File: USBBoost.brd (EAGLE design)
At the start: 43.8 x 20.3 mm, 27 parts, among them IC1 RT9276, J1 Input, J2 3.75V, J3 2.33V, J4 1.17V, J5 Status, X1 USB_

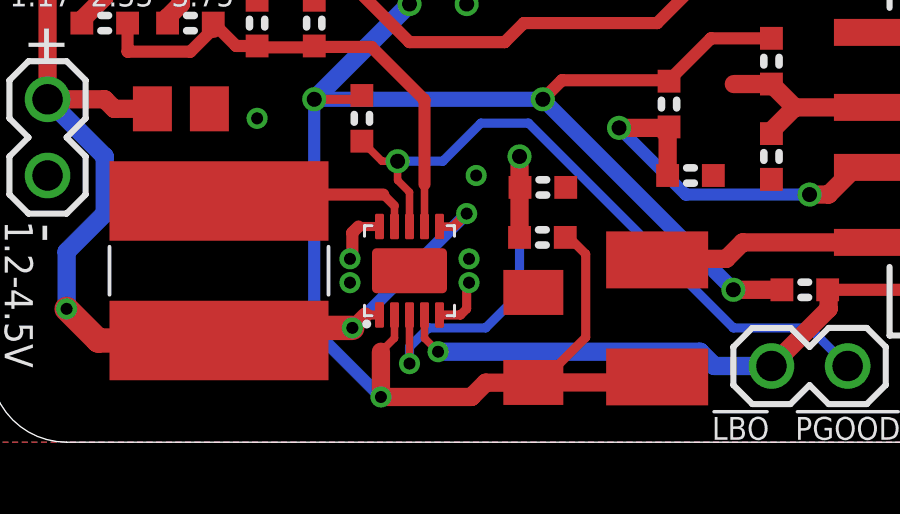
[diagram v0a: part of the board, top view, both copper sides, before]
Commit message: foo
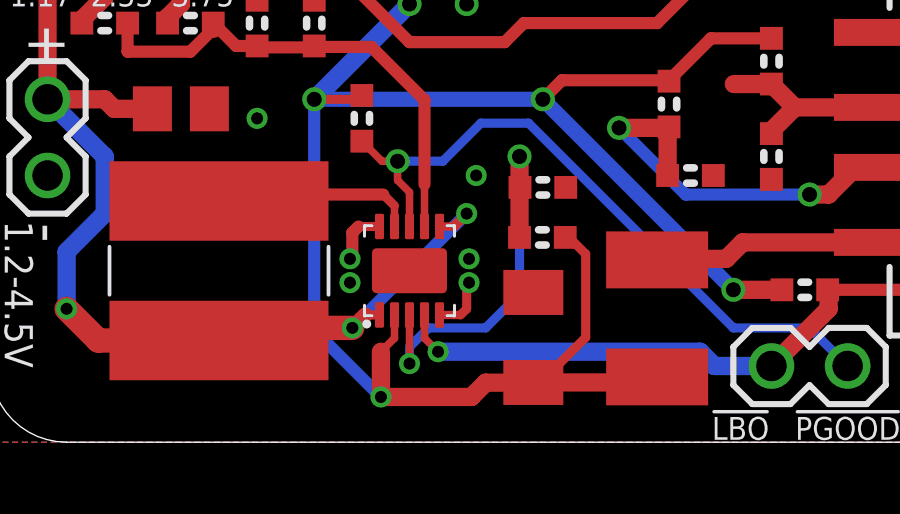
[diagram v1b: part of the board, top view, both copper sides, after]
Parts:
- removed R15: 20k0, freetronics-original:0603
- added R3: 49k9, freetronics-original:0603
- R10: value 1k -> 130k
- R11: value 130k -> 73k2
- R12: value 73k2 -> 26k7
- R13: value 26k7 -> 20k
- R14: value 20k -> 20k0
- R5: value 49k9 -> 180k
- R6: value 180k -> 10k
- R8: value 10k -> 1k
- moved R8 17.0 mm to (15.9, 17.8), turned to 90 degrees
- moved R7 15.8 mm to (27.1, 5.08), turned to 0 degrees
- moved R14 9.38 mm to (18.4, 8.49), turned to 180 degrees
- moved R5 8.10 mm to (18.4, 6.83), turned to 180 degrees
- moved R6 7.21 mm to (12.4, 10.8), turned to 270 degrees
- moved R13 6.98 mm to (10.8, 14.0), turned to 270 degrees
- moved R10 6.35 mm to (8.89, 14.0)
- moved R12 2.86 mm to (3.81, 14.0)
- moved R4 2.77 mm to (26.0, 9.53), turned to 270 degrees
- moved R11 2.22 mm to (6.67, 14.0), turned to 180 degrees
- moved R9 1.90 mm to (14.0, 17.8)
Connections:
- net !LBO: now also R7.2; no longer R8.2
- net !PGOOD: now also R6.2; no longer R7.2
- net FB: now also R14.2, R5.2; no longer R15.2, R6.2
- net GND: now also R13.1, R3.2; no longer R15.1, R5.2
- net LBI: now also R10.1, R13.2; no longer R13.1, R14.2
- net N$10: now also R4.1; no longer R5.1
- net N$11: now also R11.2; no longer R12.2
- net N$12: now also R12.2; no longer R13.2
- net N$15: now also R9.2; no longer R10.2
- net N$5: now also R10.2; no longer R11.2
- net N$7: now also R3.1; no longer R4.1
- net N$8: now also R8.2; no longer R9.2
- net VOUT: now also R5.1; no longer R10.1
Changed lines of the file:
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@@
 <elements>
 <element name="C1" library="freetronics-jon" package="C0805" value="10uF" x="6.35" y="11.1125" smashed="yes"/>
-<element name="R15" library="freetronics-original" package="0603" value="20k0" x="18.415" y="8.493125" smashed="yes" rot="R180"/>
-<element name="R6" library="freetronics-original" package="0603" value="180k" x="18.399225" y="6.82625" smashed="yes" rot="R180"/>
+<element name="R14" library="freetronics-original" package="0603" value="20k0" x="18.415" y="8.493125" smashed="yes" rot="R180"/>
+<element name="R5" library="freetronics-original" package="0603" value="180k" x="18.399225" y="6.82625" smashed="yes" rot="R180"/>
 <element name="C2" library="freetronics-jon" package="C1206K" value="22uF" x="18.0975" y="3.4924" smashed="yes" rot="R90"/>
-<element name="R9" library="freetronics-original" package="0603" value="1k" x="15.875" y="17.78" smashed="yes" rot="R90"/>
+<element name="R8" library="freetronics-original" package="0603" value="1k" x="15.875" y="17.78" smashed="yes" rot="R90"/>
 <element name="J1" library="freetronics-master-v1" package="1X02" value="Input" x="1.90495" y="11.43" smashed="yes" rot="R270"/>
 <element name="X1" library="freetronics-master-v1" package="USB-A-S-SILK-FEMALE" value="USB_" x="36.83" y="10.16" smashed="yes" rot="R180"/>
 <element name="R2" library="freetronics-original" package="0603" value="75k" x="26.035" y="12.7" smashed="yes" rot="R270"/>
-<element name="R5" library="freetronics-original" package="0603" value="49k9" x="26.035" y="9.525" smashed="yes" rot="R270"/>
+<element name="R4" library="freetronics-original" package="0603" value="49k9" x="26.035" y="9.525" smashed="yes" rot="R270"/>
 <element name="R1" library="freetronics-original" package="0603" value="75k" x="22.621875" y="11.27125" smashed="yes" rot="R270"/>
-<element name="R4" library="freetronics-original" package="0603" value="49k9" x="23.33625" y="8.89" smashed="yes"/>
+<element name="R3" library="freetronics-original" package="0603" value="49k9" x="23.33625" y="8.89" smashed="yes"/>
 <element name="LED1" library="freetronics-master-v1" package="LED-0603" value="Power" x="17.78" y="17.78" smashed="yes" rot="R270"/>
 <element name="L1" library="freetronics-luke" package="CDRH" value="6.8 uH" x="7.62" y="5.715" smashed="yes" rot="R180"/>
@@
 <element name="J3" library="freetronics-luke" package="SJ" value="2.33V" x="6.35" y="17.145" smashed="yes" rot="R90"/>
 <element name="J4" library="freetronics-luke" package="SJ" value="1.17V" x="3.81" y="17.145" smashed="yes" rot="R90"/>
-<element name="R13" library="freetronics-original" package="0603" value="26k7" x="3.81" y="13.97" smashed="yes" rot="R180"/>
-<element name="R12" library="freetronics-original" package="0603" value="73k2" x="6.6675" y="13.97" smashed="yes" rot="R180"/>
-<element name="R11" library="freetronics-original" package="0603" value="130k" x="8.89" y="13.97" smashed="yes" rot="R90"/>
-<element name="R14" library="freetronics-original" package="0603" value="20k" x="10.795" y="13.97" smashed="yes" rot="R270"/>
-<element name="R7" library="freetronics-original" package="0603" value="10k" x="12.3825" y="10.795" smashed="yes" rot="R270"/>
-<element name="R8" library="freetronics-original" package="0603" value="10k" x="27.14625" y="5.08" smashed="yes"/>
-<element name="R10" library="freetronics-original" package="0603" value="1k" x="13.97" y="17.78" smashed="yes" rot="R90"/>
+<element name="R12" library="freetronics-original" package="0603" value="26k7" x="3.81" y="13.97" smashed="yes" rot="R180"/>
+<element name="R11" library="freetronics-original" package="0603" value="73k2" x="6.6675" y="13.97" smashed="yes" rot="R180"/>
+<element name="R10" library="freetronics-original" package="0603" value="130k" x="8.89" y="13.97" smashed="yes" rot="R90"/>
+<element name="R13" library="freetronics-original" package="0603" value="20k" x="10.795" y="13.97" smashed="yes" rot="R270"/>
+<element name="R6" library="freetronics-original" package="0603" value="10k" x="12.3825" y="10.795" smashed="yes" rot="R270"/>
+<element name="R7" library="freetronics-original" package="0603" value="10k" x="27.14625" y="5.08" smashed="yes"/>
+<element name="R9" library="freetronics-original" package="0603" value="1k" x="13.97" y="17.78" smashed="yes" rot="R90"/>
 <element name="LED2" library="freetronics-master-v1" package="LED-0603" value="Low Batt" x="12.065" y="17.78" smashed="yes" rot="R270"/>
 <element name="J5" library="freetronics-master-v1" package="1X02" value="Status" x="28.575" y="2.54" smashed="yes" rot="R180"/>
@@
 <signal name="GND">
 <contactref element="C1" pad="2"/>
-<contactref element="R15" pad="1"/>
+<contactref element="R14" pad="1"/>
 <contactref element="C2" pad="2"/>
-<contactref element="R5" pad="2"/>
 <contactref element="R4" pad="2"/>
+<contactref element="R3" pad="2"/>
 <contactref element="LED1" pad="C"/>
 <polygon width="0.4064" layer="1" isolate="0.4064">
@@
 <vertex x="-0.635" y="0"/>
 </polygon>
-<contactref element="R14" pad="1"/>
+<contactref element="R13" pad="1"/>
 <contactref element="J1" pad="2"/>
 <contactref element="X1" pad="GND"/>
@@
 <via x="10.795" y="15.875" extent="1-16" drill="0.5"/>
 <via x="15.875" y="14.605" extent="1-16" drill="0.5"/>
-<wire x1="14.97" y1="4.24" x2="15.67" y2="4.24" width="0.3048" layer="1"/>
+<wire x1="14.97" y1="4.24" x2="15.67" y2="4.24" width="0.2794" layer="1"/>
 <wire x1="15.67" y1="4.24" x2="15.875" y2="4.445" width="0.3048" layer="1"/>
 <wire x1="15.875" y1="4.445" x2="15.875" y2="5.23875" width="0.3048" layer="1"/>
@@
 </signal>
 <signal name="FB">
-<contactref element="R6" pad="2"/>
-<contactref element="R15" pad="2"/>
+<contactref element="R5" pad="2"/>
+<contactref element="R14" pad="2"/>
 <contactref element="IC1" pad="3"/>
 <wire x1="13.97" y1="4.24" x2="13.97" y2="2.619375" width="0.254" layer="1"/>
@@
 </signal>
 <signal name="N$8">
-<contactref element="R9" pad="2"/>
+<contactref element="R8" pad="2"/>
 <contactref element="LED1" pad="A"/>
 <wire x1="15.875" y1="18.542" x2="17.78" y2="18.542" width="0.4064" layer="1"/>
@@
 </signal>
 <signal name="VOUT">
-<contactref element="R6" pad="1"/>
-<contactref element="R9" pad="1"/>
+<contactref element="R5" pad="1"/>
+<contactref element="R8" pad="1"/>
 <contactref element="C2" pad="1"/>
 <contactref element="R2" pad="1"/>
 <contactref element="R1" pad="1"/>
 <contactref element="F1" pad="1"/>
+<contactref element="R6" pad="1"/>
 <contactref element="R7" pad="1"/>
-<contactref element="R8" pad="1"/>
-<contactref element="R10" pad="1"/>
+<contactref element="R9" pad="1"/>
 <contactref element="IC1" pad="2"/>
 <wire x1="13.47" y1="4.24" x2="13.47" y2="3.46875" width="0.254" layer="1"/>
@@
 <signal name="N$7">
 <contactref element="R1" pad="2"/>
-<contactref element="R4" pad="1"/>
+<contactref element="R3" pad="1"/>
 <contactref element="X1" pad="D-"/>
 <via x="27.305" y="8.255" extent="1-16" drill="0.5"/>
@@
 <signal name="N$10">
 <contactref element="R2" pad="2"/>
-<contactref element="R5" pad="1"/>
+<contactref element="R4" pad="1"/>
 <contactref element="X1" pad="D+"/>
 <wire x1="29.618" y1="11.16" x2="26.813" y2="11.16" width="0.6096" layer="1"/>
@@
 <signal name="N$5">
 <contactref element="J2" pad="1"/>
-<contactref element="R11" pad="2"/>
+<contactref element="R10" pad="2"/>
 <wire x1="8.89" y1="14.732" x2="8.89" y2="16.383" width="0.6096" layer="1"/>
 </signal>
 <signal name="N$11">
 <contactref element="J3" pad="1"/>
-<contactref element="R12" pad="2"/>
+<contactref element="R11" pad="2"/>
 <wire x1="5.9055" y1="13.97" x2="5.9055" y2="14.1605" width="0.6096" layer="1"/>
 <wire x1="5.9055" y1="14.1605" x2="6.35" y2="14.605" width="0.6096" layer="1"/>
@@
 <signal name="N$12">
 <contactref element="J4" pad="1"/>
-<contactref element="R13" pad="2"/>
+<contactref element="R12" pad="2"/>
 <wire x1="3.048" y1="13.97" x2="3.048" y2="14.081125" width="0.6096" layer="1"/>
 <wire x1="3.048" y1="14.081125" x2="3.81" y2="14.843125" width="0.6096" layer="1"/>
@@
 </signal>
 <signal name="!PGOOD">
-<contactref element="R7" pad="2"/>
+<contactref element="R6" pad="2"/>
 <contactref element="J5" pad="1"/>
 <contactref element="IC1" pad="8"/>
@@
 </signal>
 <signal name="!LBO">
-<contactref element="R8" pad="2"/>
+<contactref element="R7" pad="2"/>
 <contactref element="LED2" pad="C"/>
 <contactref element="J5" pad="2"/>
@@
 </signal>
 <signal name="N$15">
-<contactref element="R10" pad="2"/>
+<contactref element="R9" pad="2"/>
 <contactref element="LED2" pad="A"/>
 <wire x1="12.065" y1="18.542" x2="13.97" y2="18.542" width="0.4064" layer="1"/>
 </signal>
 <signal name="LBI">
+<contactref element="R10" pad="1"/>
+<contactref element="R12" pad="1"/>
+<contactref element="R13" pad="2"/>
 <contactref element="R11" pad="1"/>
-<contactref element="R13" pad="1"/>
-<contactref element="R14" pad="2"/>
-<contactref element="R12" pad="1"/>
 <wire x1="8.937625" y1="13.160375" x2="8.89" y2="13.208" width="0.4064" layer="1"/>
 <contactref element="IC1" pad="7"/>
